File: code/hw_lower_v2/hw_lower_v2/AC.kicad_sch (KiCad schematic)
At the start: 38 parts, among them K1 AHES4191, Q1 BSS138, Q2 BSS138, Q3 BSS138, T1 TS3193-2C 2mA/2mA, U1 BRCS02C, U2 BL0942

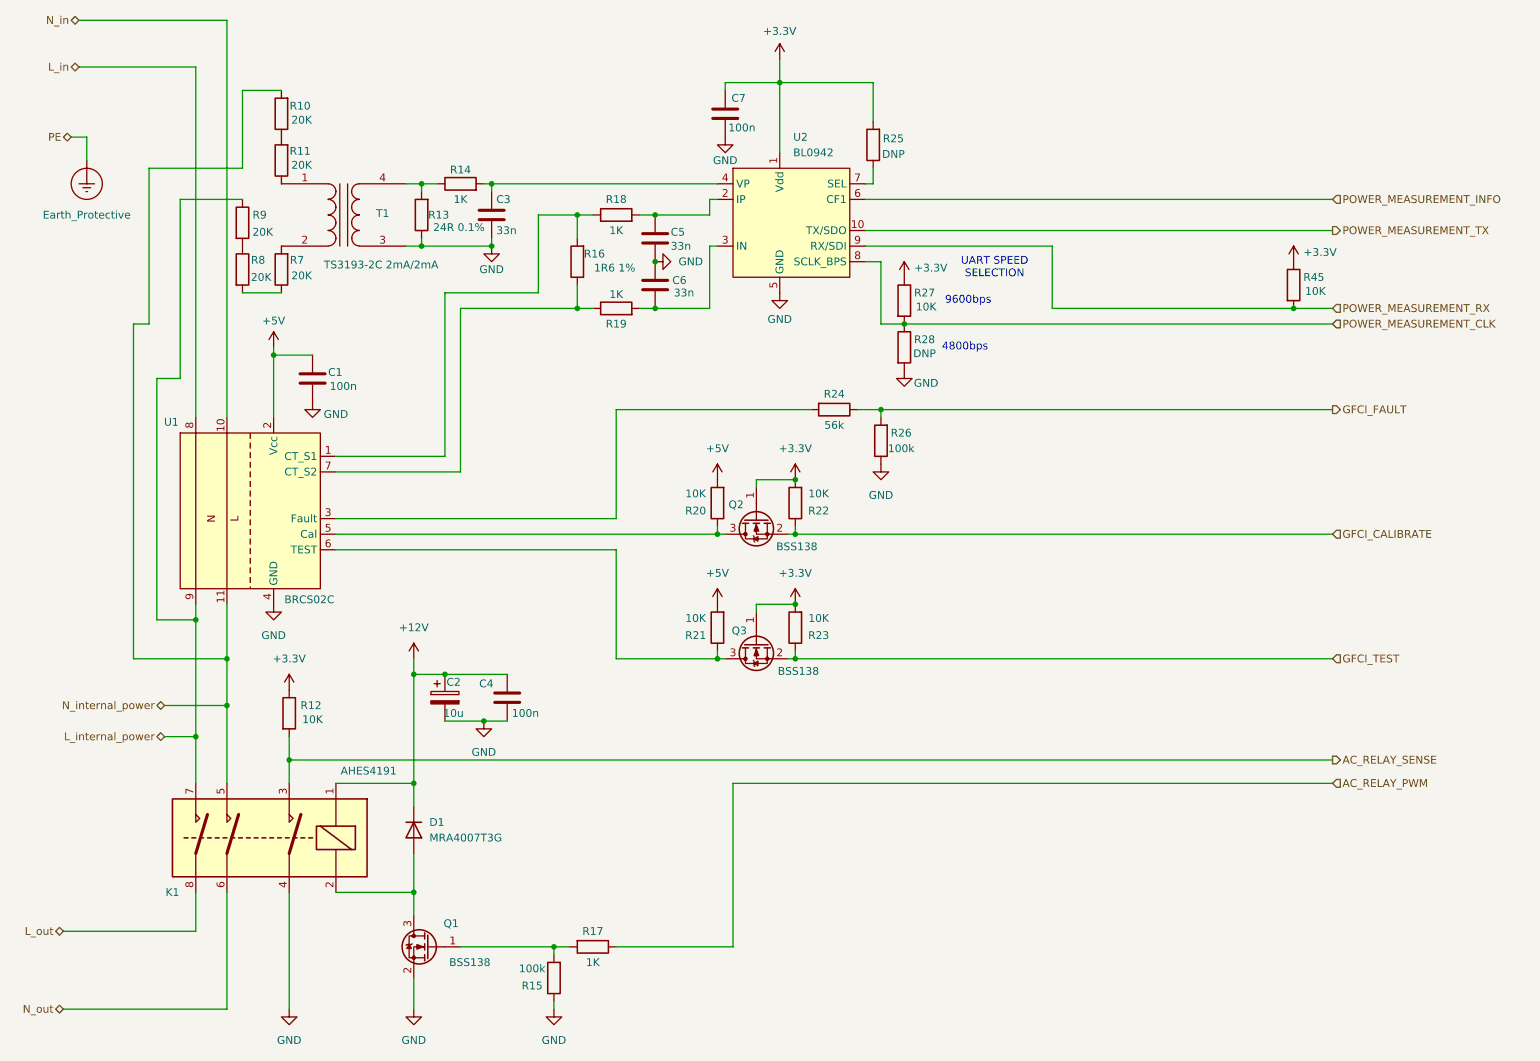
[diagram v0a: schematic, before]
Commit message: commit before experimenting
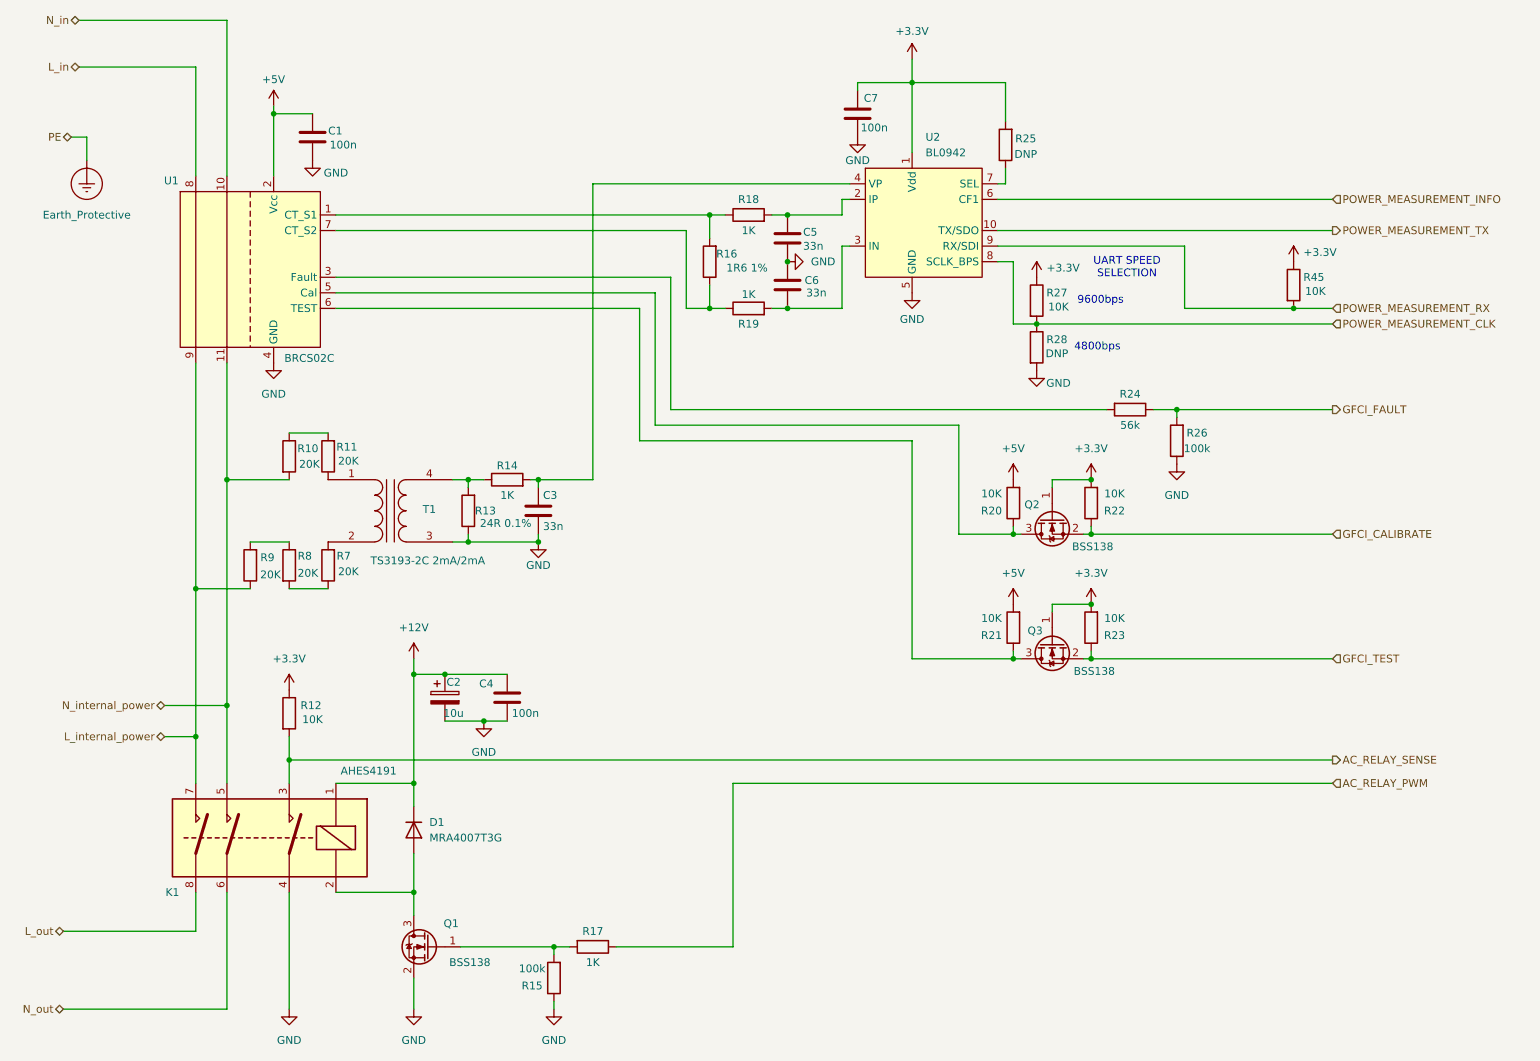
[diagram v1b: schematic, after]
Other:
- moved on the sheet: C1, C3, C5, C6, C7, Q2, Q3, R10, R11, R13, R14, R16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

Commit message: have one project part library
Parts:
- U2: footprint JLCPCB:SSOP-10_L4.9-W3.9-P1.00-LS6.0-BL -> multi_new:SSOP-10_L4.9-W3.9-P1.00-LS6.0-BL
